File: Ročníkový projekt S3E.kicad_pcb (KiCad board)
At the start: 2 copper layers, 116.3 x 113 mm, 101 parts, among them IC1 PIC18F47Q43-I_P, IC2 ULN2804A, IC3 L7805CD2T-TR, IC4 MCP7940M-I_SN, J1 DG126-5.0-02P-14-00A, J2 DS1021-1_2SF11-B, J3 DS1021-1_2SF11-B, J4 TSW-105-07-G-S, J5 DS1021-1_2SF11-B, J6 DS1021-1_2SF11-B, J7 DS1021-1_2SF11-B, J8 DS1021-1_2SF11-B, Q1 DTA123JCAT116, Q2 DTA123JCAT116, Q3 DTA123JCAT116, Q4 DTA123JCAT116, Q5 DTA123JCAT116, Q6 DTA123JCAT116, Y1 32 768Hz

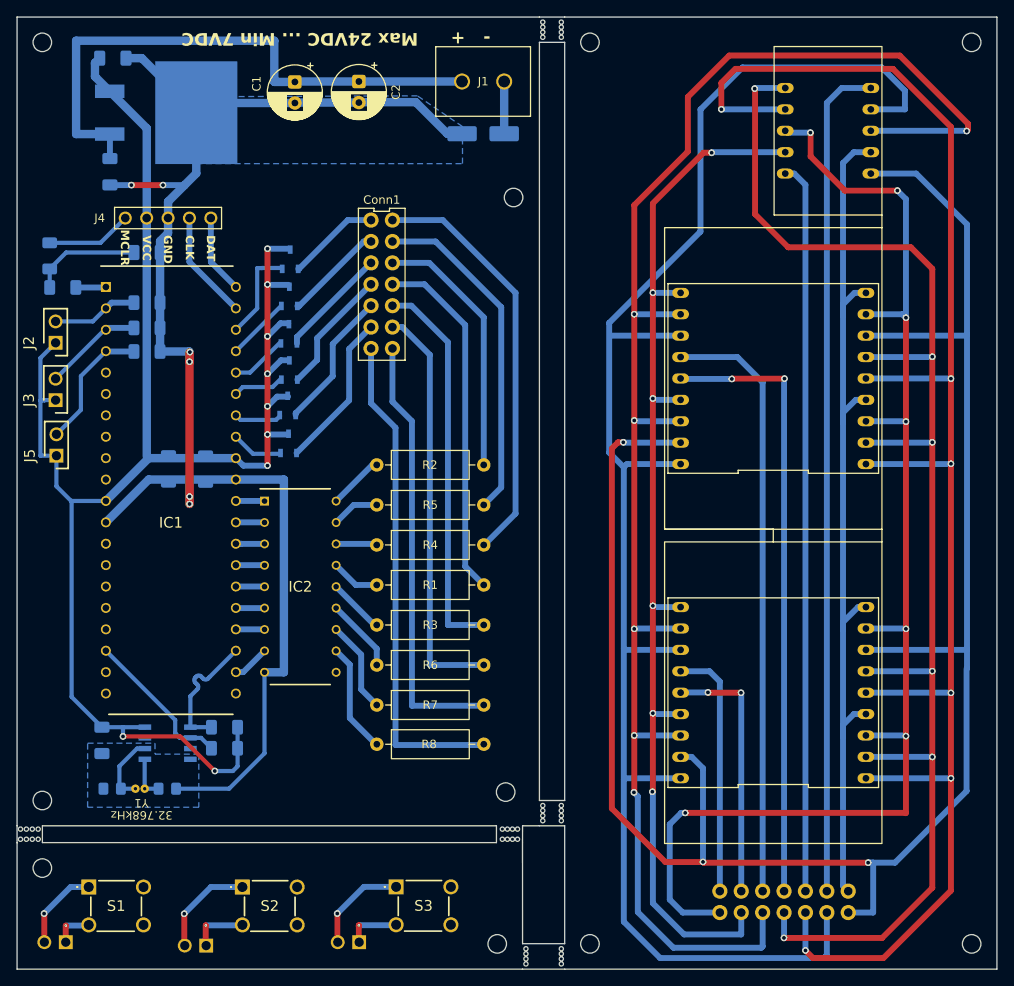
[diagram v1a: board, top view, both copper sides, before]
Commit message: Auto-backup: 10:53:27 17/04/2026
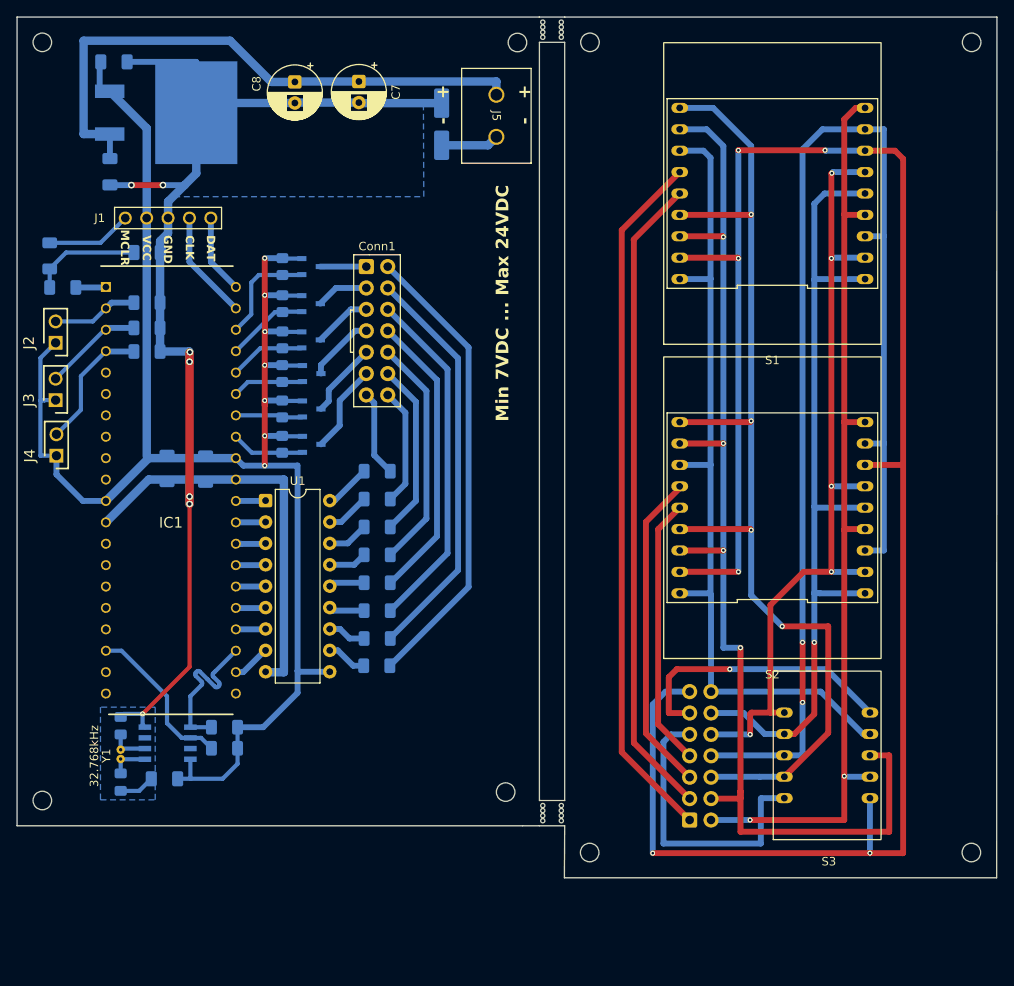
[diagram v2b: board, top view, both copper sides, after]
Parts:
- removed the ? at (125.8, 150.7)
- removed the ? at (130.0, 152.5)
- removed the ? at (123.0, 137.7)
- removed the ? at (124.2, 136.5)
- removed the ? at (67.2, 136.5)
- removed the ? at (125.8, 151.3)
- removed the ? at (125.8, 151.9)
- removed the ? at (130.0, 151.3)
- removed the ? at (124.2, 137.7)
- removed the ? at (66.5, 136.5)
- removed the ? at (65.8, 136.5)
- removed the ? at (130.0, 151.9)
- removed the ? at (66.5, 137.7)
- removed the ? at (124.8, 136.5)
- removed the ? at (123.0, 136.5)
- removed the ? at (67.9, 136.5)
- removed the ? at (130.0, 150.7)
- removed the ? at (124.8, 137.7)
- removed the ? at (68.4, 141.1)
- removed the ? at (67.2, 137.7)
- removed the ? at (123.6, 137.7)
- removed the ? at (65.8, 137.7)
- removed the ? at (125.8, 152.5)
- removed the ? at (67.9, 137.7)
- removed the ? at (123.6, 136.5)
- removed the ? at (122.4, 150.1)
- removed the C10 at (75.4, 126.0)
- removed the IC2 at (99.0, 107.7)
- removed the J1 at (118.2, 47.8)
- removed J6, J7, J8: DS1021-1_2SF11-B, SamacSys_Parts:HDRV2W64P0X254_1X2_508X254X588P
- removed the R1 at (108.1, 107.5)
- removed the R2 at (108.1, 93.3)
- removed the R3 at (108.1, 112.3)
- removed the R4 at (108.1, 102.8)
- removed the R5 at (108.1, 98.0)
- removed the S1 at (73.9, 143.4)
- removed the S1 at (155.1, 120.3)
- added C4: 100nF, Capacitor_SMD:C_1206_3216Metric_Pad1.33x1.80mm_HandSolder, B.Cu at (82.9, 130.5)
- added J5: DG126-5.0-02P-14-00A, My parts:CONN_DG126-5.0-02P_DEG, F.Cu at (122.3, 49.3)
- added R10: 220R, Resistor_SMD:R_1206_3216Metric_Pad1.30x1.75mm_HandSolder, B.Cu at (108.1, 100.6)
- added R11: 220R, Resistor_SMD:R_1206_3216Metric_Pad1.30x1.75mm_HandSolder, B.Cu at (108.1, 97.3)
- added R12: 220R, Resistor_SMD:R_1206_3216Metric_Pad1.30x1.75mm_HandSolder, B.Cu at (108.1, 94.0)
- added R13: 220R, Resistor_SMD:R_1206_3216Metric_Pad1.30x1.75mm_HandSolder, B.Cu at (108.1, 117.1)
- added R16: 10K, Resistor_SMD:R_0805_2012Metric_Pad1.20x1.40mm_HandSolder, B.Cu at (96.8, 90.8)
- added R17: 10K, Resistor_SMD:R_0805_2012Metric_Pad1.20x1.40mm_HandSolder, B.Cu at (96.8, 86.6)
- added R18: 10K, Resistor_SMD:R_0805_2012Metric_Pad1.20x1.40mm_HandSolder, B.Cu at (96.8, 82.4)
- added R19: 10K, Resistor_SMD:R_0805_2012Metric_Pad1.20x1.40mm_HandSolder, B.Cu at (96.9, 78.4)
- added R20: 10K, Resistor_SMD:R_0805_2012Metric_Pad1.20x1.40mm_HandSolder, B.Cu at (96.9, 74.1)
- added R21: 10K, Resistor_SMD:R_0805_2012Metric_Pad1.20x1.40mm_HandSolder, B.Cu at (96.9, 69.7)
- added R9: 220R, Resistor_SMD:R_1206_3216Metric_Pad1.30x1.75mm_HandSolder, B.Cu at (108.1, 104.0)
- added S1: ~, My parts:DIP 18 Patice Display Digit 1, F.Cu at (155.0, 61.1)
- added U1: ULN2803A, Package_DIP:DIP-18_W7.62mm, F.Cu at (94.9, 97.5)
- C5: renamed from C9; value 7pF -> 6,8pF
- C6: renamed from C8; value 7pF -> 6,8pF
- Q1, Q2, Q3, Q4, Q5, Q6: value DTA123JCAT116 -> YJL2301D; footprint My parts:TRANS_DTA113ZCAH_ROM -> My parts:SOT95P240X115-3N
- R15: value 4k7 -> 4K7
- R6, R7, R8: value 330R -> 220R; footprint Resistor_THT:R_Axial_DIN0309_L9.0mm_D3.2mm_P12.70mm_Horizontal -> Resistor_SMD:R_1206_3216Metric_Pad1.30x1.75mm_HandSolder; moved to B.Cu
- S2: value TACT-67N-F -> ~; footprint My parts:TACT67NF -> My parts:DIP 18 Patice Display Digit 1
- S3: value TACT-67N-F -> ~; footprint My parts:TACT67NF -> My parts:DIP-10 Patice Display Digit 3 4
- moved S2 77.4 mm to (155.0, 98.4), turned to 90 degrees
- moved S3 53.5 mm to (161.5, 127.8), turned to 90 degrees
- moved Q6 21.2 mm to (100.3, 69.7), turned to 0 degrees
- moved Conn2 20.0 mm to (146.5, 127.8), turned to 90 degrees
- moved R8 19.2 mm to (108.1, 107.3)
- moved H3 18.4 mm to (124.8, 43.1)
- moved R7 11.2 mm to (108.1, 110.6)
- moved ? 10.8 mm to (133.3, 139.3)
- moved H6 10.8 mm to (178.6, 139.3)
- moved Q4 9.88 mm to (100.3, 78.4), turned to 0 degrees
- moved Q2 9.32 mm to (100.3, 86.6), turned to 0 degrees
- moved C6 7.55 mm to (77.7, 124.2), turned to -90 degrees
- moved C5 5.59 mm to (77.7, 130.9), turned to -90 degrees
- moved Conn1 5.55 mm to (108.1, 77.4)
- moved Q1 5.43 mm to (100.3, 90.8), turned to 0 degrees
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- renumbered C5 to C1, C4 to C10, C7 to C2, C6 to C3, C2 to C7, C1 to C8, C3 to C9, IC4 to IC2, J4 to J1, J5 to J4, R12 to R1, R10 to R2, R11 to R3, R9 to R4, R13 to R5
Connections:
- Conn1 pad 1: DIGIT_6 -> /Display_Board/D6
- Conn1 pad 10: E' -> /D'
- Conn1 pad 11: D' -> /C'
- Conn1 pad 12: A' -> /B'
- Conn1 pad 13: B' -> /A'
- Conn1 pad 14: C' -> /DP'
- Conn1 pad 2: DIGIT_5 -> /Display_Board/D5
- Conn1 pad 3: DIGIT_4 -> /Display_Board/D4
- Conn1 pad 4: DIGIT_3 -> /Display_Board/D3
- Conn1 pad 5: DIGIT_2 -> /Display_Board/D2
- Conn1 pad 6: DIGIT_1 -> /Display_Board/D1
- Conn1 pad 7: DP' -> /G'
- Conn1 pad 8: G' -> /F'
- Conn1 pad 9: F' -> /E'
- Conn2 pad 1: DIGIT_6 -> /Display_Board/D6
- Conn2 pad 10: E' -> /D'
- Conn2 pad 11: D' -> /C'
- Conn2 pad 12: A' -> /B'
- Conn2 pad 13: B' -> /A'
- Conn2 pad 14: C' -> /DP'
- Conn2 pad 2: DIGIT_5 -> /Display_Board/D5
- Conn2 pad 3: DIGIT_4 -> /Display_Board/D4
- Conn2 pad 4: DIGIT_3 -> /Display_Board/D3
- Conn2 pad 5: DIGIT_2 -> /Display_Board/D2
- Conn2 pad 6: DIGIT_1 -> /Display_Board/D1
- Conn2 pad 7: DP' -> /G'
- Conn2 pad 8: G' -> /F'
- Conn2 pad 9: F' -> /E'
- IC2 pad 4: VCC_P -> VDD_P
- IC2 pad 8: VDD_P -> VCC_P
- Q1 pad 1: DIGIT_2 -> A_1
- Q1 pad 2: A_2 -> VCC_P
- Q1 pad 3: VCC_P -> /Display_Board/D1
- Q2 pad 1: DIGIT_4 -> A_2
- Q2 pad 2: A_4 -> VCC_P
- Q2 pad 3: VCC_P -> /Display_Board/D2
- Q3 pad 1: DIGIT_3 -> A_3
- Q3 pad 2: A_3 -> VCC_P
- Q3 pad 3: VCC_P -> /Display_Board/D3
- Q4 pad 1: DIGIT_6 -> A_4
- Q4 pad 2: A_6 -> VCC_P
- Q4 pad 3: VCC_P -> /Display_Board/D4
- Q5 pad 1: DIGIT_5 -> A_5
- Q5 pad 2: A_5 -> VCC_P
- Q5 pad 3: VCC_P -> /Display_Board/D5
- Q6 pad 1: DIGIT_1 -> A_6
- Q6 pad 2: A_1 -> VCC_P
- Q6 pad 3: VCC_P -> /Display_Board/D6
- R6 pad 1: /F -> /A
- R6 pad 2: F' -> /A'
- R7 pad 1: /G -> /B
- R7 pad 2: G' -> /B'
- R8 pad 1: /DP -> /C
- R8 pad 2: DP' -> /C'
- S2 pad 1: /Buttons_board/Button_2 -> /E'
- S2 pad 2: unconnected-(S3-Pad2) -> /D'
- S2 pad 3: VCC_P -> /C'
- S2 pad 4: unconnected-(S3-Pad4) -> /DP'
- S3 pad 1: /Buttons_board/Button_3 -> /G'
- S3 pad 2: unconnected-(S4-Pad2) -> /DP'
- S3 pad 3: VCC_P -> /A'
- S3 pad 4: unconnected-(S4-Pad4) -> /F'
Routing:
- net G': track 280.6 -> 0.00 mm, vias 3 -> 0
- net F': track 244.4 -> 0.00 mm
- net E': track 244.2 -> 0.00 mm, vias 6 -> 0
- net /G': track 0.00 -> 240.1 mm, vias 0 -> 6
- net A': track 224.3 -> 0.00 mm, vias 6 -> 0
- net D': track 212.9 -> 0.00 mm, vias 6 -> 0
- net C': track 205.3 -> 0.00 mm, vias 7 -> 0
- net /A': track 0.00 -> 186.8 mm, vias 0 -> 4
- net /C': track 0.00 -> 184.8 mm, vias 0 -> 2
- net /B': track 0.00 -> 170.2 mm, vias 0 -> 4
- net B': track 169.8 -> 0.00 mm, vias 6 -> 0
- net /DP': track 0.00 -> 167.8 mm, vias 0 -> 2
- net DP': track 167.5 -> 0.00 mm
- net /D': track 0.00 -> 123.9 mm, vias 0 -> 5
- net /E': track 0.00 -> 120.4 mm, vias 0 -> 1
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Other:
- board size 116.3 x 113 mm -> 116.3 x 102.2 mm
- board text added: "Min 7VDC ... Max 24VDC"
- board text removed: "Max 24VDC ... Min 7VDC"
